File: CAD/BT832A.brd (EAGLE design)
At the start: 24.9 x 50 mm, 43 parts, among them IC1 CP2102, U1 MCP73831T-3ACI/OT, U2 BT832, U3 LP5907MFX-3.3/NOPB, U4 LP5907MFX-3.3/NOPB, U5 ADS131M08IPBS, U6 BCM857BS, X1 ABM3B-8.000MHZ-B2-T, X2 FC-12M

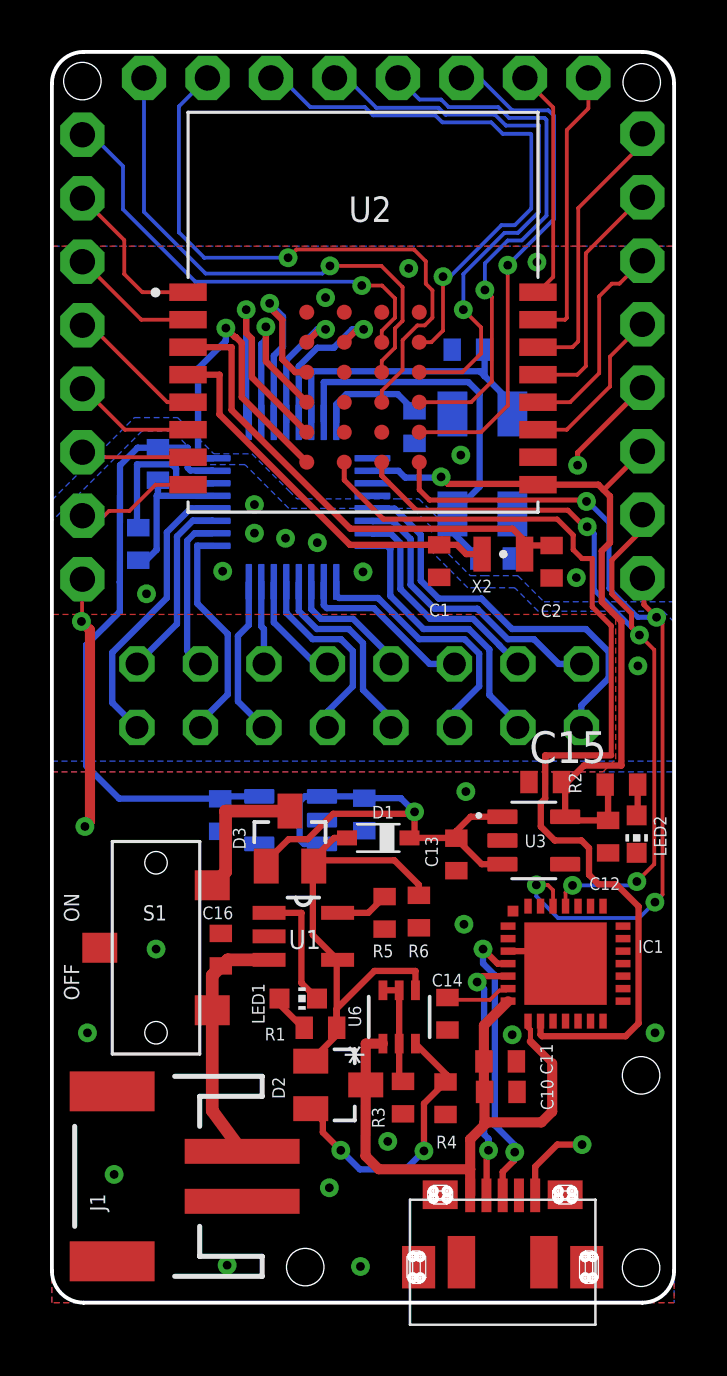
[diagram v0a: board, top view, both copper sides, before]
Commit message: Update BT832A.brd
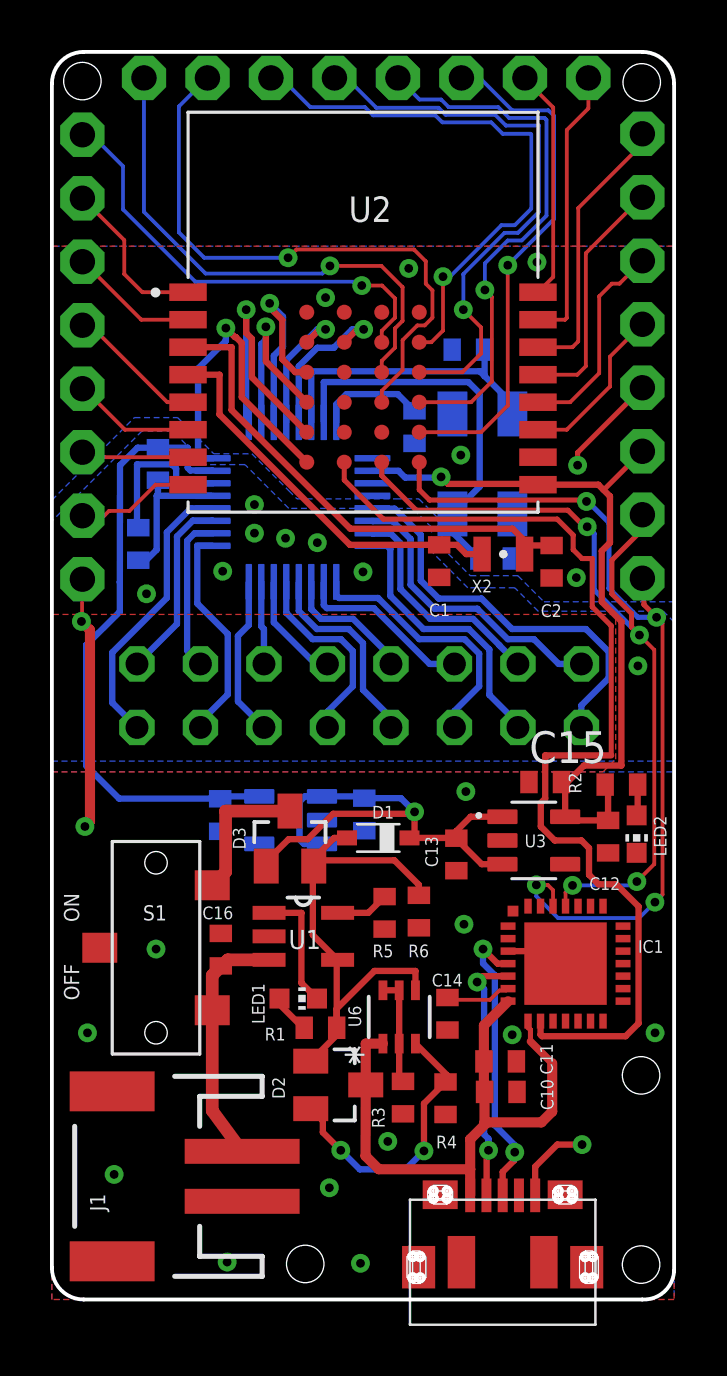
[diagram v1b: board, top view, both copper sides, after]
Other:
- board size 24.9 x 50 mm -> 24.9 x 49.9 mm
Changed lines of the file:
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@@
 ADC inputs may have to be a (CHEAP) SMT connector backside to minimize possible interference from the radio,
 but let's just break them out first and test. Let's still ID a 16-20 pin connector.</text>
-<wire x1="6.604" y1="-27.94" x2="6.604" y2="19.558" width="0.1524" layer="20"/>
+<wire x1="6.604" y1="-27.813" x2="6.604" y2="19.558" width="0.1524" layer="20"/>
 <wire x1="6.604" y1="19.558" x2="7.874" y2="20.828" width="0.1524" layer="20" curve="-90"/>
 <wire x1="7.874" y1="20.828" x2="30.226" y2="20.828" width="0.1524" layer="20"/>
 <wire x1="30.226" y1="20.828" x2="31.496" y2="19.558" width="0.1524" layer="20" curve="-90"/>
 <wire x1="31.496" y1="19.558" x2="31.496" y2="-27.94" width="0.1524" layer="20"/>
-<wire x1="31.496" y1="-27.94" x2="30.226" y2="-29.21" width="0.1524" layer="20" curve="-90"/>
-<wire x1="30.226" y1="-29.21" x2="7.874" y2="-29.21" width="0.1524" layer="20"/>
-<wire x1="7.874" y1="-29.21" x2="6.604" y2="-27.94" width="0.1524" layer="20" curve="-90"/>
-<dimension x1="38.862" y1="20.828" x2="31.75" y2="-29.21" x3="36.83" y3="-4.191" textsize="1.778" layer="47" dtype="vertical"/>
+<wire x1="31.496" y1="-27.94" x2="30.226" y2="-29.083" width="0.1524" layer="20" curve="-90"/>
+<wire x1="30.226" y1="-29.083" x2="7.874" y2="-29.083" width="0.1524" layer="20"/>
+<wire x1="7.874" y1="-29.083" x2="6.604" y2="-27.813" width="0.1524" layer="20" curve="-90"/>
 <dimension x1="6.604" y1="19.558" x2="31.496" y2="18.796" x3="19.05" y3="23.114" textsize="1.778" layer="47" dtype="horizontal"/>
 <hole x="30.2006" y="19.6088" drill="1.5"/>
 <hole x="7.8232" y="19.6596" drill="1.5"/>
-<hole x="30.1752" y="-27.813" drill="1.5"/>
-<hole x="16.7386" y="-27.7876" drill="1.5"/>
+<hole x="30.1752" y="-27.686" drill="1.5"/>
+<hole x="16.7386" y="-27.6606" drill="1.5"/>
 <hole x="30.1752" y="-20.1168" drill="1.5"/>
 <text x="11.2014" y="-13.3096" size="0.6096" layer="21" rot="R180">S1</text>
@@
  JACOB TINKHAUSER
       MIT LICENSE</text>
+<dimension x1="31.496" y1="-29.083" x2="29.464" y2="20.828" x3="34.5186" y3="-4.1275" textsize="1.778" layer="47" dtype="vertical"/>
 </plain>
 <attributes>
@@
 <vertex x="6.604" y="-7.9756"/>
 <vertex x="31.496" y="-7.9756"/>
-<vertex x="31.496" y="-29.21"/>
-<vertex x="6.604" y="-29.21"/>
+<vertex x="31.496" y="-29.083"/>
+<vertex x="6.604" y="-29.083"/>
 </polygon>
 <polygon width="0.1524" layer="16">
@@
 </polygon>
 <polygon width="0.1524" layer="1">
-<vertex x="6.604" y="-29.21"/>
+<vertex x="6.604" y="-29.083"/>
 <vertex x="6.604" y="-7.9756"/>
 <vertex x="28.6512" y="-7.9756"/>
@@
 <vertex x="6.604" y="13.0556"/>
 <vertex x="31.496" y="13.0556"/>
-<vertex x="31.496" y="-29.21"/>
+<vertex x="31.496" y="-29.083"/>
 </polygon>
 <via x="27.6352" y="4.2926" extent="1-16" drill="0.35"/>
@@
 <via x="8.0264" y="-18.415" extent="1-16" drill="0.35"/>
 <via x="9.0932" y="-24.0792" extent="1-16" drill="0.35"/>
-<via x="13.6144" y="-27.7114" extent="1-16" drill="0.35"/>
+<via x="13.6144" y="-27.5844" extent="1-16" drill="0.35"/>
 <via x="17.7038" y="-24.6126" extent="1-16" drill="0.35"/>
 <via x="27.813" y="-22.8854" extent="1-16" drill="0.35"/>
@@
 <contactref element="C14" pad="1"/>
 <contactref element="C15" pad="1"/>
-<via x="18.9484" y="-27.7622" extent="1-16" drill="0.35"/>
+<via x="18.9484" y="-27.6352" extent="1-16" drill="0.35"/>
 <contactref element="U$1" pad="MP1"/>
 <contactref element="U$1" pad="MP2"/>
@@
 <wire x1="9.0932" y1="-24.0792" x2="13.3604" y2="-14.4376" width="0" layer="19" extent="1-1"/>
 <wire x1="14.2156" y1="-25.1554" x2="9.0932" y2="-24.0792" width="0" layer="19" extent="1-1"/>
-<wire x1="13.6144" y1="-27.7114" x2="14.2156" y2="-25.1554" width="0" layer="19" extent="1-1"/>
+<wire x1="13.6144" y1="-27.5844" x2="14.2156" y2="-25.1554" width="0" layer="19" extent="1-1"/>
 <wire x1="17.7038" y1="-24.6126" x2="14.2156" y2="-25.1554" width="0" layer="19" extent="1-1"/>
 <wire x1="20.0406" y1="-22.7584" x2="17.7038" y2="-24.6126" width="0" layer="19" extent="1-1"/>
@@
 <wire x1="26.288" y1="-27.5914" x2="25.938" y2="-24.9164" width="0" layer="19" extent="1-1"/>
 <wire x1="22.988" y1="-27.5914" x2="26.288" y2="-27.5914" width="0" layer="19" extent="1-1"/>
-<wire x1="18.9484" y1="-27.7622" x2="17.7038" y2="-24.6126" width="0" layer="19" extent="1-1"/>
+<wire x1="18.9484" y1="-27.6352" x2="17.7038" y2="-24.6126" width="0" layer="19" extent="1-1"/>
 <wire x1="19.1008" y1="-10.3274" x2="19.9644" y2="-14.2136" width="0" layer="19" extent="1-16"/>
 <wire x1="17.4094" y1="-9.906" x2="19.1008" y2="-10.3274" width="0" layer="19" extent="16-16"/>
